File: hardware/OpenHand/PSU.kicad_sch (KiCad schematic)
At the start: 0 parts

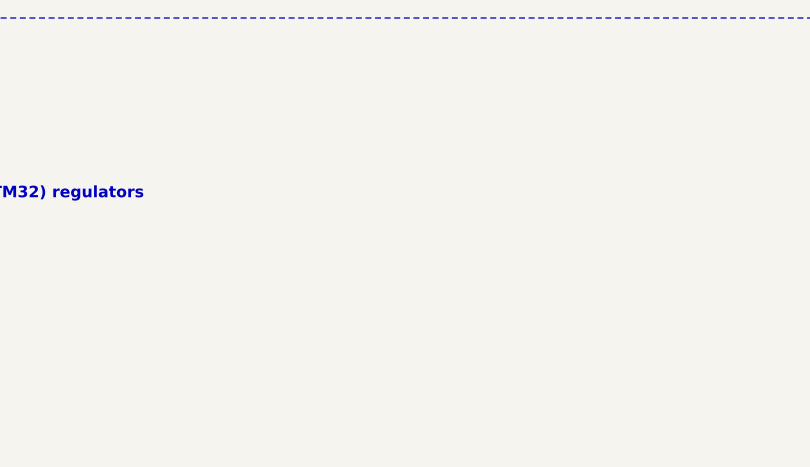
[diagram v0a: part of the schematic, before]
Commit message: working on schematics
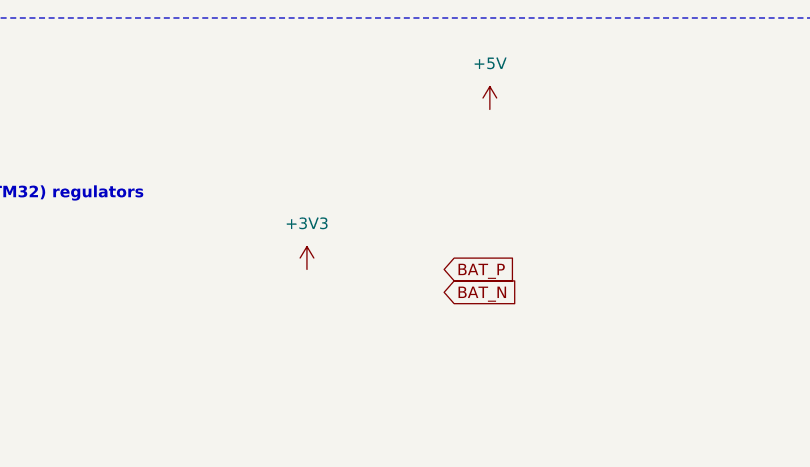
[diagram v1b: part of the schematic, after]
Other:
- title: (none) -> OpenHand prosthetic hand controller project
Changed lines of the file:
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@@
 (kicad_sch (version 20230121) (generator eeschema)
   (paper "A4")
+  (title_block
+    (title "OpenHand prosthetic hand controller project")
+    (date "2024-01-31")
+    (rev "v1.0")
+    (comment 1 "Aleksa Heler")
+  )
   (rectangle (start 22.86 88.9) (end 170.18 190.5)
     (stroke (width 0) (type dash_dot))
@@
     (effects (font (size 1.27 1.27) bold) (justify left bottom))
   )
+  (global_label "BAT_N" (shape input) (at 104.14 53.34 0) (fields_autoplaced)
+    (effects (font (size 1.27 1.27)) (justify left))
+    (property "Intersheetrefs" "${INTERSHEET_REFS}" (at 112.7495 53.34 0)
+      (effects (font (size 1.27 1.27)) (justify left) hide)
+    )
+  )
+  (global_label "BAT_P" (shape input) (at 104.14 50.8 0) (fields_autoplaced)
+    (effects (font (size 1.27 1.27)) (justify left))
+    (property "Intersheetrefs" "${INTERSHEET_REFS}" (at 112.689 50.8 0)
+      (effects (font (size 1.27 1.27)) (justify left) hide)
+    )
+  )
+  (symbol (lib_id "power:+5V") (at 109.22 33.02 0) (unit 1)
+    (in_bom yes) (on_board yes) (dnp no) (fields_autoplaced)
+    (property "Reference" "#PWR01" (at 109.22 36.83 0)
+      (effects (font (size 1.27 1.27)) hide)
+    )
+    (property "Value" "+5V" (at 109.22 27.94 0)
+      (effects (font (size 1.27 1.27)))
+    )
+    (property "Footprint" "" (at 109.22 33.02 0)
+      (effects (font (size 1.27 1.27)) hide)
+    )
+    (property "Datasheet" "" (at 109.22 33.02 0)
+      (effects (font (size 1.27 1.27)) hide)
+    )
+    (pin "1")
+    (instances
+      (project "OpenHand"
+        (path "/f1fbd835-8408-4592-854c-2fbec9d052ec"
+          (reference "#PWR01") (unit 1)
+        )
+        (path "/f1fbd835-8408-4592-854c-2fbec9d052ec/11b37193-b902-4bf9-977f-96c37af6f134"
+          (reference "#PWR028") (unit 1)
+        )
+      )
+    )
+  )
+  (symbol (lib_id "power:+3V3") (at 88.9 50.8 0) (unit 1)
+    (in_bom yes) (on_board yes) (dnp no) (fields_autoplaced)
+    (property "Reference" "#PWR040" (at 88.9 54.61 0)
+      (effects (font (size 1.27 1.27)) hide)
+    )
+    (property "Value" "+3V3" (at 88.9 45.72 0)
+      (effects (font (size 1.27 1.27)))
+    )
+    (property "Footprint" "" (at 88.9 50.8 0)
+      (effects (font (size 1.27 1.27)) hide)
+    )
+    (property "Datasheet" "" (at 88.9 50.8 0)
+      (effects (font (size 1.27 1.27)) hide)
+    )
+    (pin "1")
+    (instances
+      (project "OpenHand"
+        (path "/f1fbd835-8408-4592-854c-2fbec9d052ec/286dde41-8068-419e-b7de-6276970410d8"
+          (reference "#PWR040") (unit 1)
+        )
+        (path "/f1fbd835-8408-4592-854c-2fbec9d052ec"
+          (reference "#PWR041") (unit 1)
+        )
+        (path "/f1fbd835-8408-4592-854c-2fbec9d052ec/11b37193-b902-4bf9-977f-96c37af6f134"
+          (reference "#PWR029") (unit 1)
+        )
+      )
+    )
+  )
 )
